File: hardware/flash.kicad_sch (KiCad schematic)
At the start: 12 parts, among them U1 ECP5U_12_CABGA256, U11 W25Q128JVS

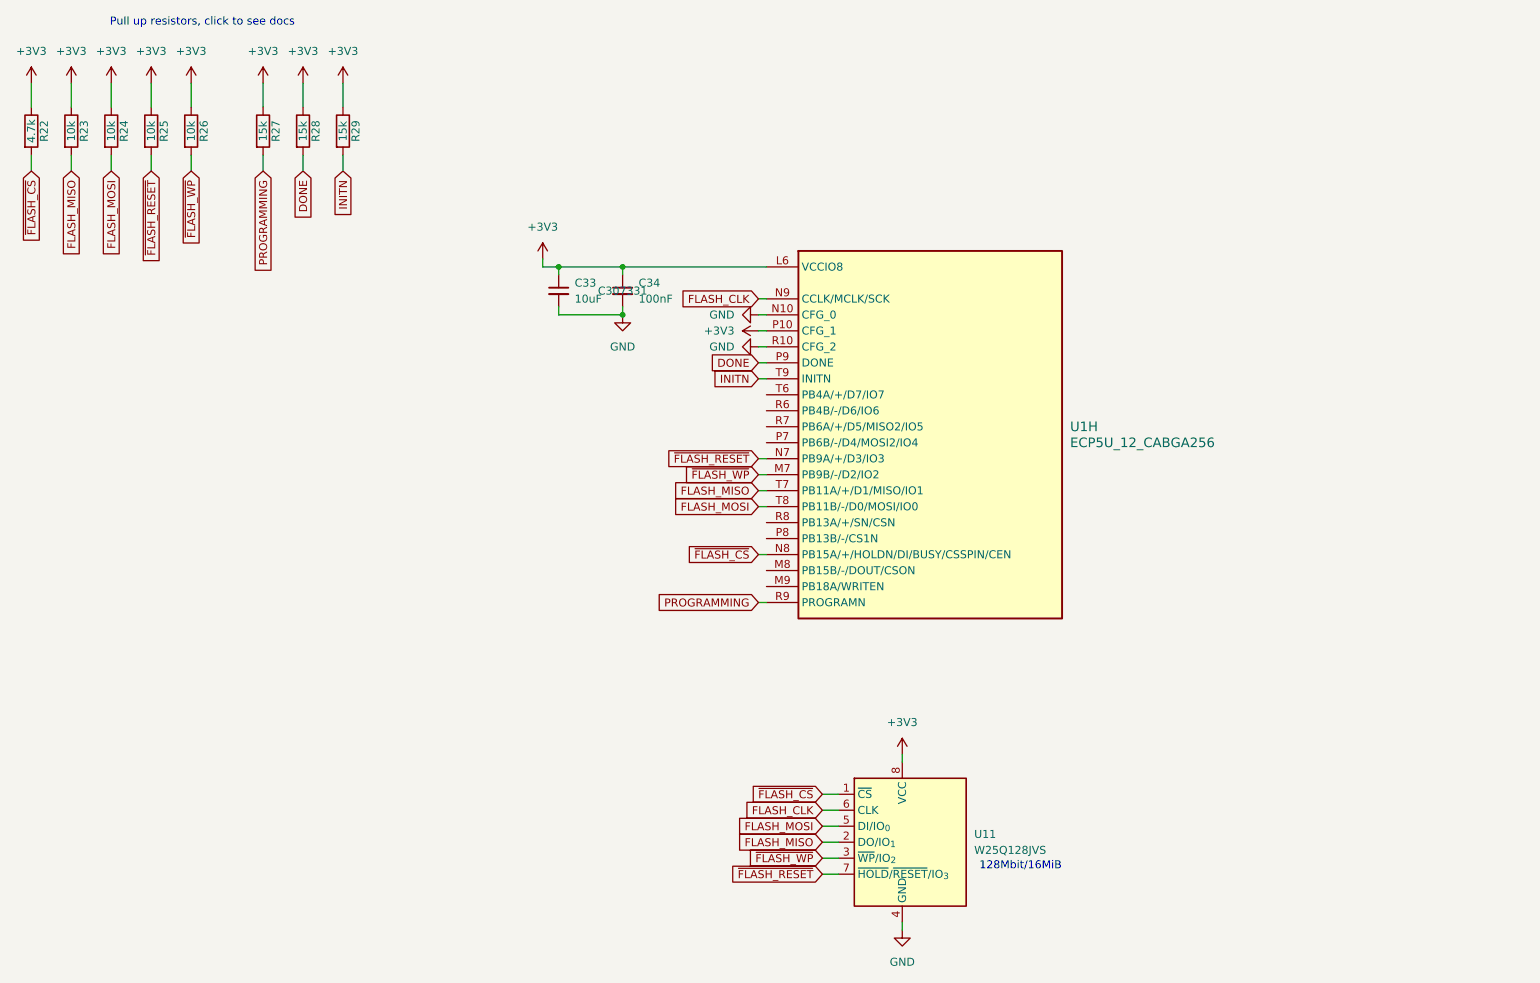
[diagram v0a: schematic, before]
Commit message: V1.0 Final Revision and Readme documentation
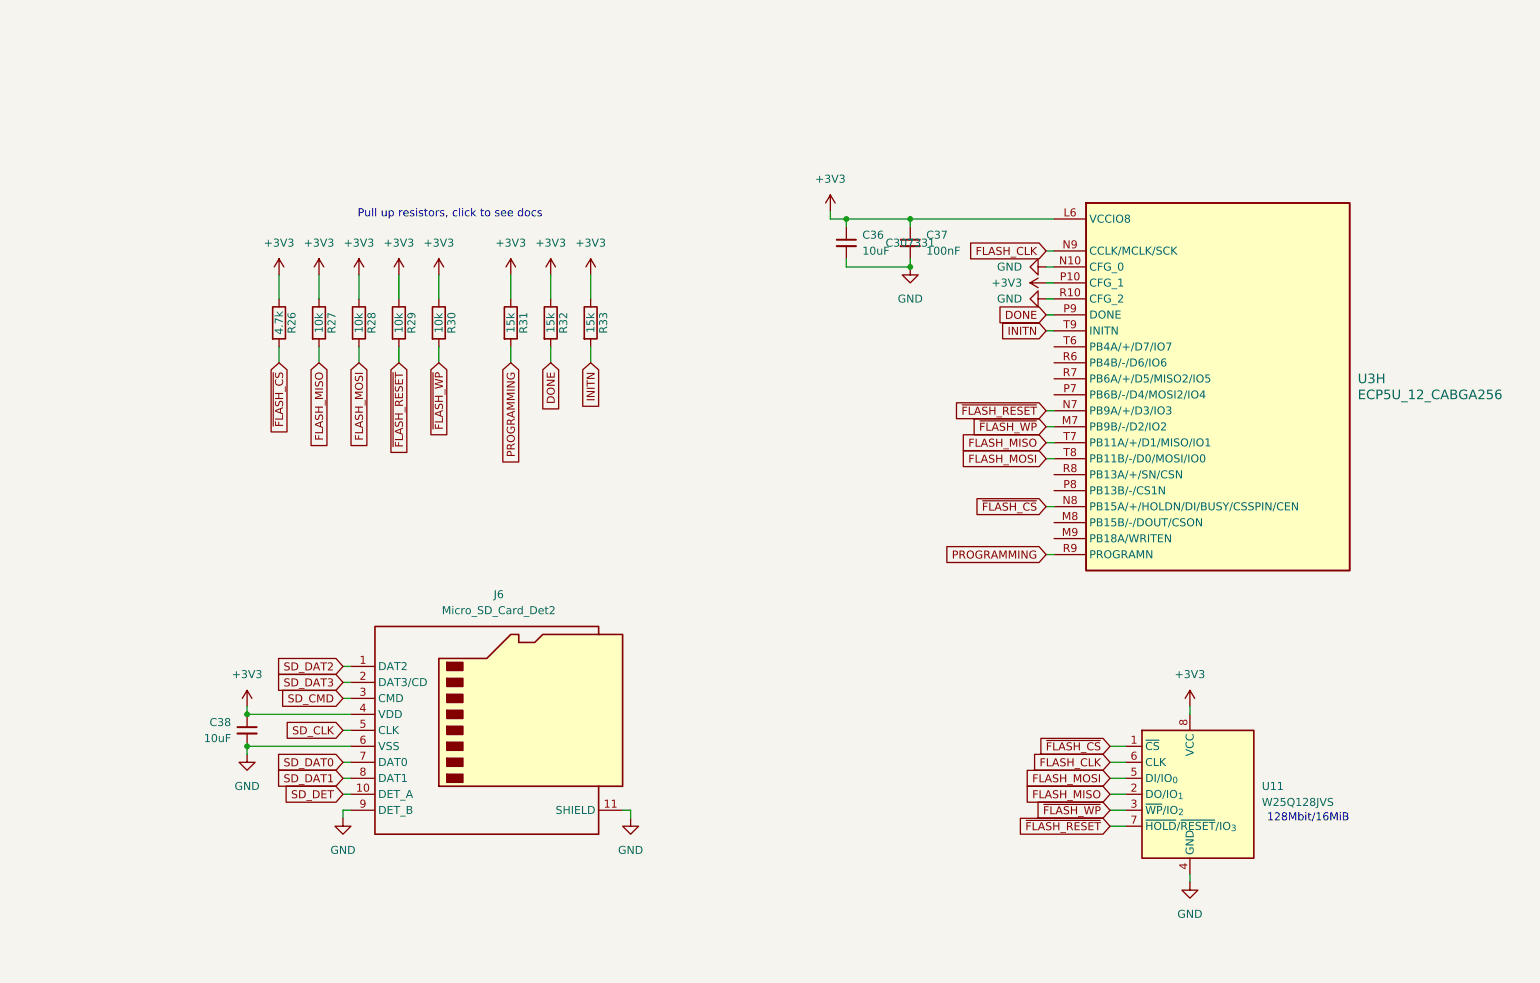
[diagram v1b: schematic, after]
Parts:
- added C38: 10uF, Capacitor_SMD:C_0603_1608Metric, symbol Device:C_Small
- added J6: Micro_SD_Card_Det2, icepi-lib:microSD_HC_SOFNG_TF-008, symbol Connector:Micro_SD_Card_Det2
- renumbered C33 to C36, C34 to C37, R22 to R26, R23 to R27, R24 to R28, R25 to R29, R26 to R30, R27 to R31, R28 to R32, R29 to R33, U1 to U3
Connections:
- net +3V3: now also C38.1, J6.4 (VDD)
- net GND: now also C38.2, J6.11 (SHIELD), J6.6 (VSS), J6.9 (DET_B)
- new net SD_CLK: J6.5 (CLK)
- new net SD_CMD: J6.3 (CMD)
- new net SD_DAT0: J6.7 (DAT0)
- new net SD_DAT1: J6.8 (DAT1)
- new net SD_DAT2: J6.1 (DAT2)
- new net SD_DAT3: J6.2 (DAT3/CD)
- new net SD_DET: J6.10 (DET_A)
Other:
- moved on the sheet: C36, C37, R26, R27, R28, R29, R30, R31, R32, R33, U11, U3H
